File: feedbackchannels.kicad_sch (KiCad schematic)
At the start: 96 parts

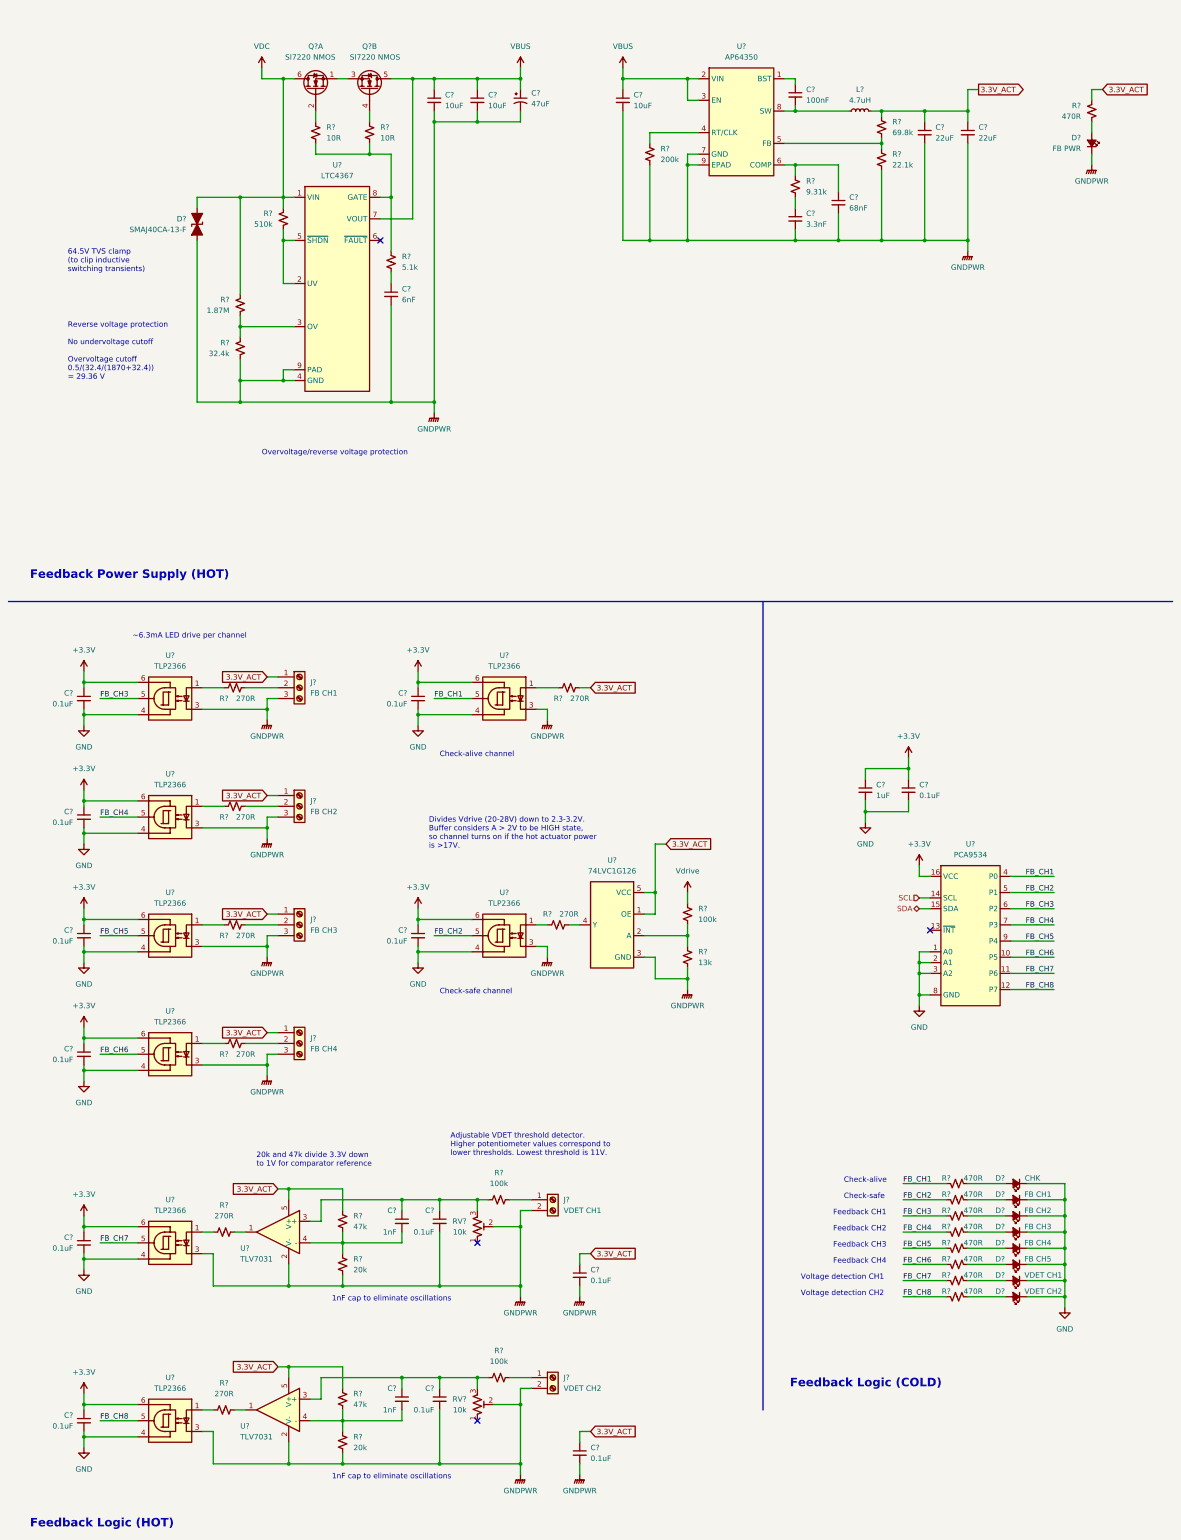
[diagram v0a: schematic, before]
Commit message: Reorganizing schematic
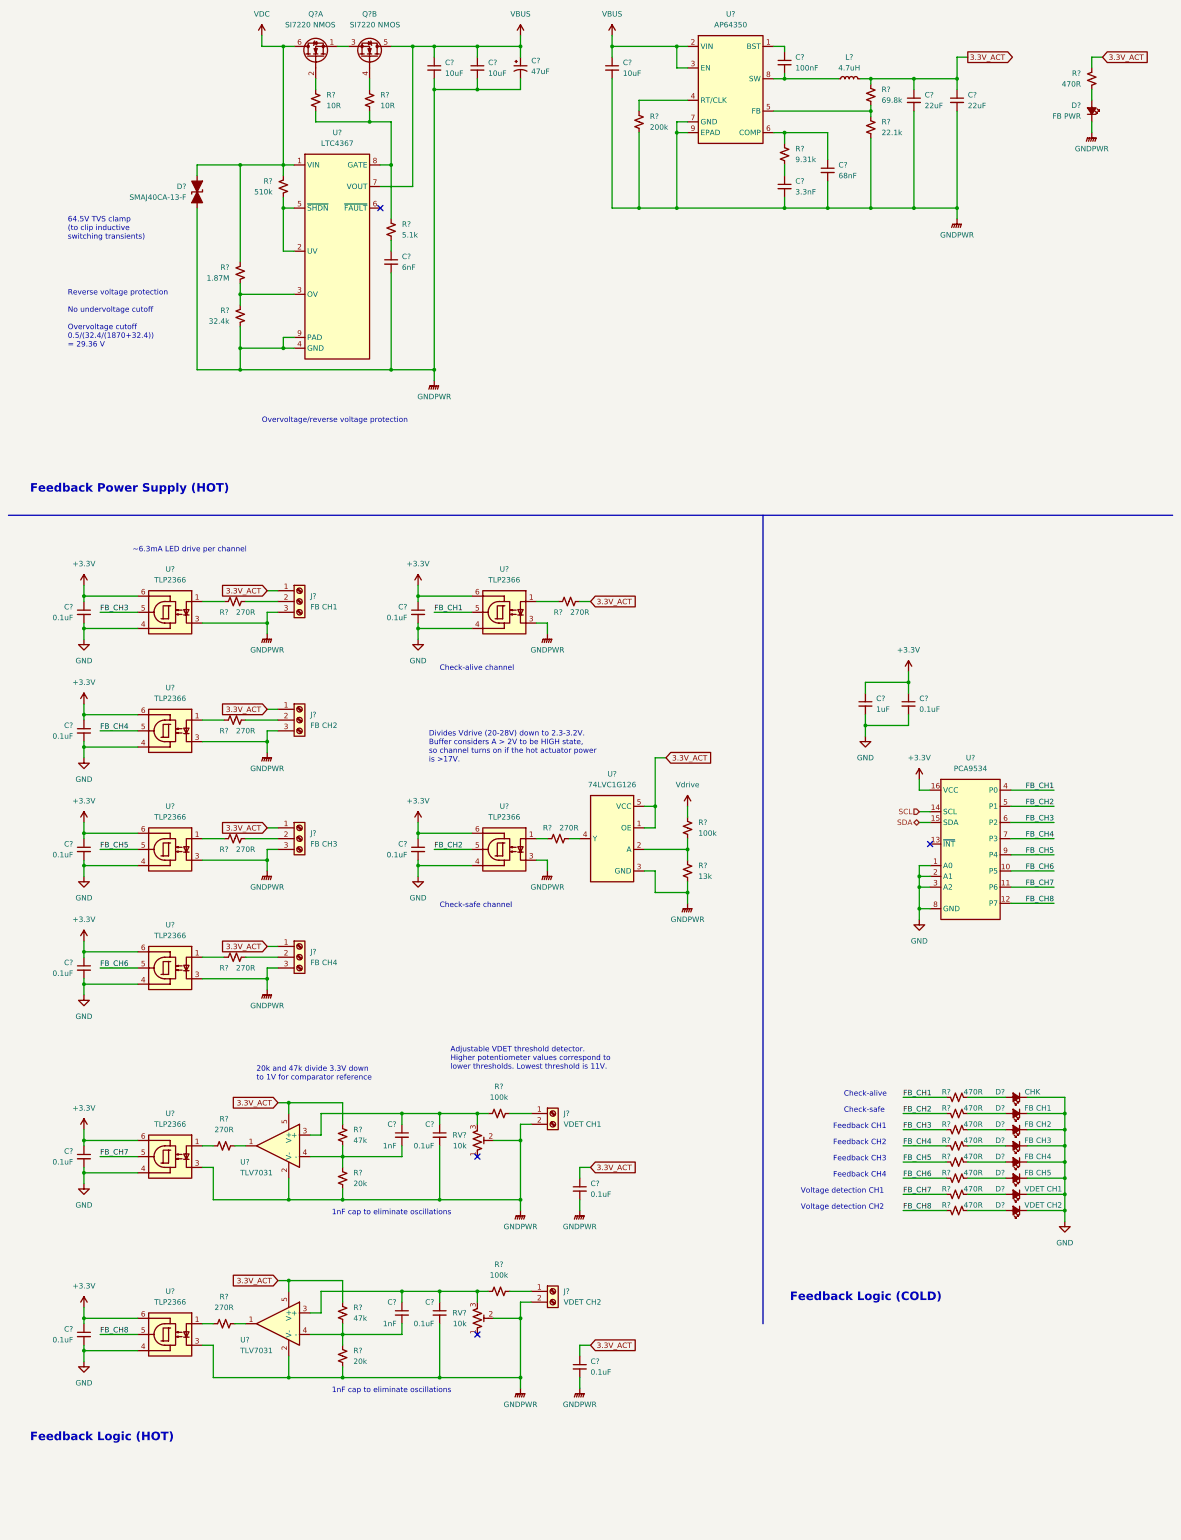
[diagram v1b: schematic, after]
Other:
- moved on the sheet: C?, D?, J?, L?, Q?A, Q?B, R?, RV?, U?
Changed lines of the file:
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@@
 (kicad_sch (version 20211123) (generator eeschema)
-  (paper "User" 299.999 399.999)
+  (paper "User" 299.999 380.009)
